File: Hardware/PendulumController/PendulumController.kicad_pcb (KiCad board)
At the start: 2 copper layers, 152 x 89 mm, 48 parts, among them J101 MOTOR, J102 ENCODER, J201 Tag Connect, J301 19V Input, J401 USB_B_Micro, J402 PROG, SW201 RESET, SW202 START_SW, SW203 STOP/MODE_SW, U201 ATmega328P-A, U301 NCV1117ST50T3G, U401 FT232RL, Y201 16mHz

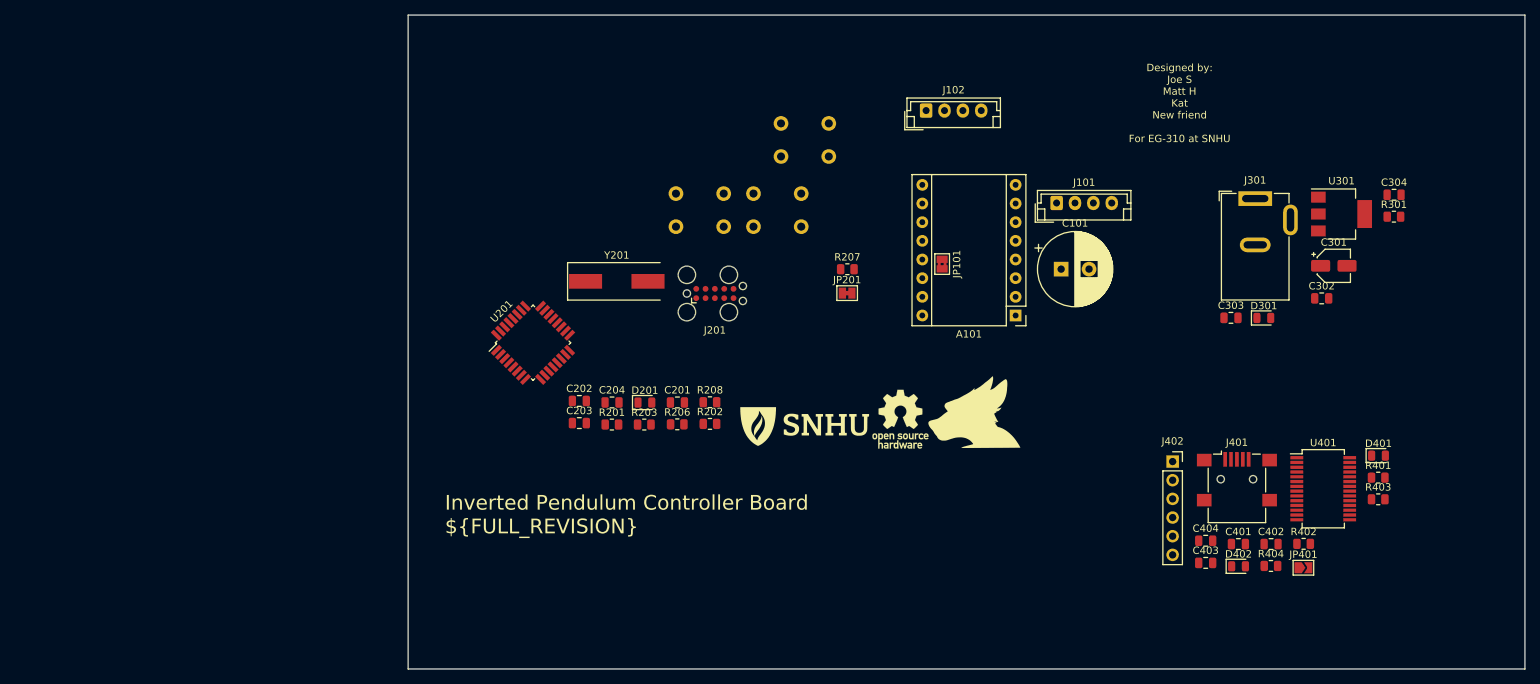
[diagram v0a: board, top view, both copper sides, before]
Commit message: Cleanup board layout, cleanup firmware and go to bed, this is a sturdy place to start a new project!
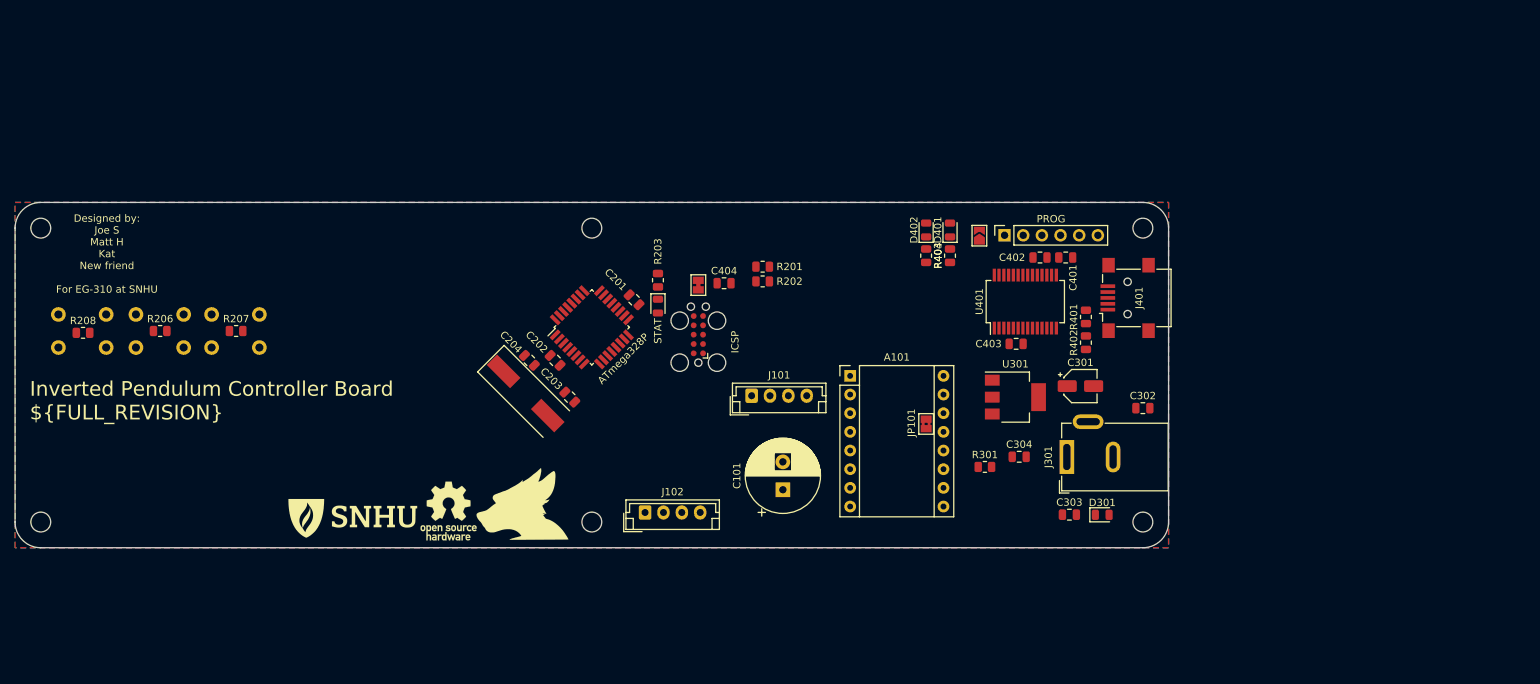
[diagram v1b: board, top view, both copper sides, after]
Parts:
- added H101: PiMountingHole, MountingHole:MountingHole_2.7mm, F.Cu at (220.0, 70.0)
- added H102: PiMountingHole, MountingHole:MountingHole_2.7mm, F.Cu at (145.0, 110.0)
- added H103: PiMountingHole, MountingHole:MountingHole_2.7mm, F.Cu at (145.0, 70.0)
- added H104: PiMountingHole, MountingHole:MountingHole_2.7mm, F.Cu at (220.0, 110.0)
- added H105: PiMountingHole, MountingHole:MountingHole_2.7mm, F.Cu at (70.0, 70.0)
- added H106: PiMountingHole, MountingHole:MountingHole_2.7mm, F.Cu at (70.0, 110.0)
- J201: value Tag Connect -> ICSP
- U201: value ATmega328P-A -> ATmega328P
- moved R208 85.9 mm to (75.8, 84.2)
- moved SW201 85.6 mm to (89.5, 81.8)
- moved SW203 85.6 mm to (78.9, 81.8)
- moved R207 83.6 mm to (96.6, 84.0)
- moved SW202 81.7 mm to (99.8, 81.8)
- moved C404 74.3 mm to (163.0, 77.5)
- moved R206 71.5 mm to (86.2, 84.0)
- moved R403 67.1 mm to (193.8, 73.8), turned to 90 degrees
- moved J102 66.7 mm to (152.2, 108.7)
- moved D401 65.9 mm to (193.8, 70.2), turned to 90 degrees
- moved R301 65.3 mm to (198.5, 102.5)
- moved JP401 63.1 mm to (197.8, 71.0), turned to 90 degrees
- moved R404 63.1 mm to (190.5, 73.8), turned to -90 degrees
- moved G*** 62.8 mm to (135.5, 107.5)
- moved REF** 62.8 mm to (125.5, 108.5)
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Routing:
- added copper zone on B.Cu, net GND
- added copper zone on F.Cu, net GND
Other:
- board size 152 x 89 mm -> 157 x 47 mm
